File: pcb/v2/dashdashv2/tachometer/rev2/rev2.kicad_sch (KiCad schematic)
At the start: 182 parts, among them Q1 BSS138, Q2 BSS138, Q3 BSS138, Q4 BSS138, Q5 BSS138, Q6 BSS138, Q7 BSS138, U1 SK6812SIDE

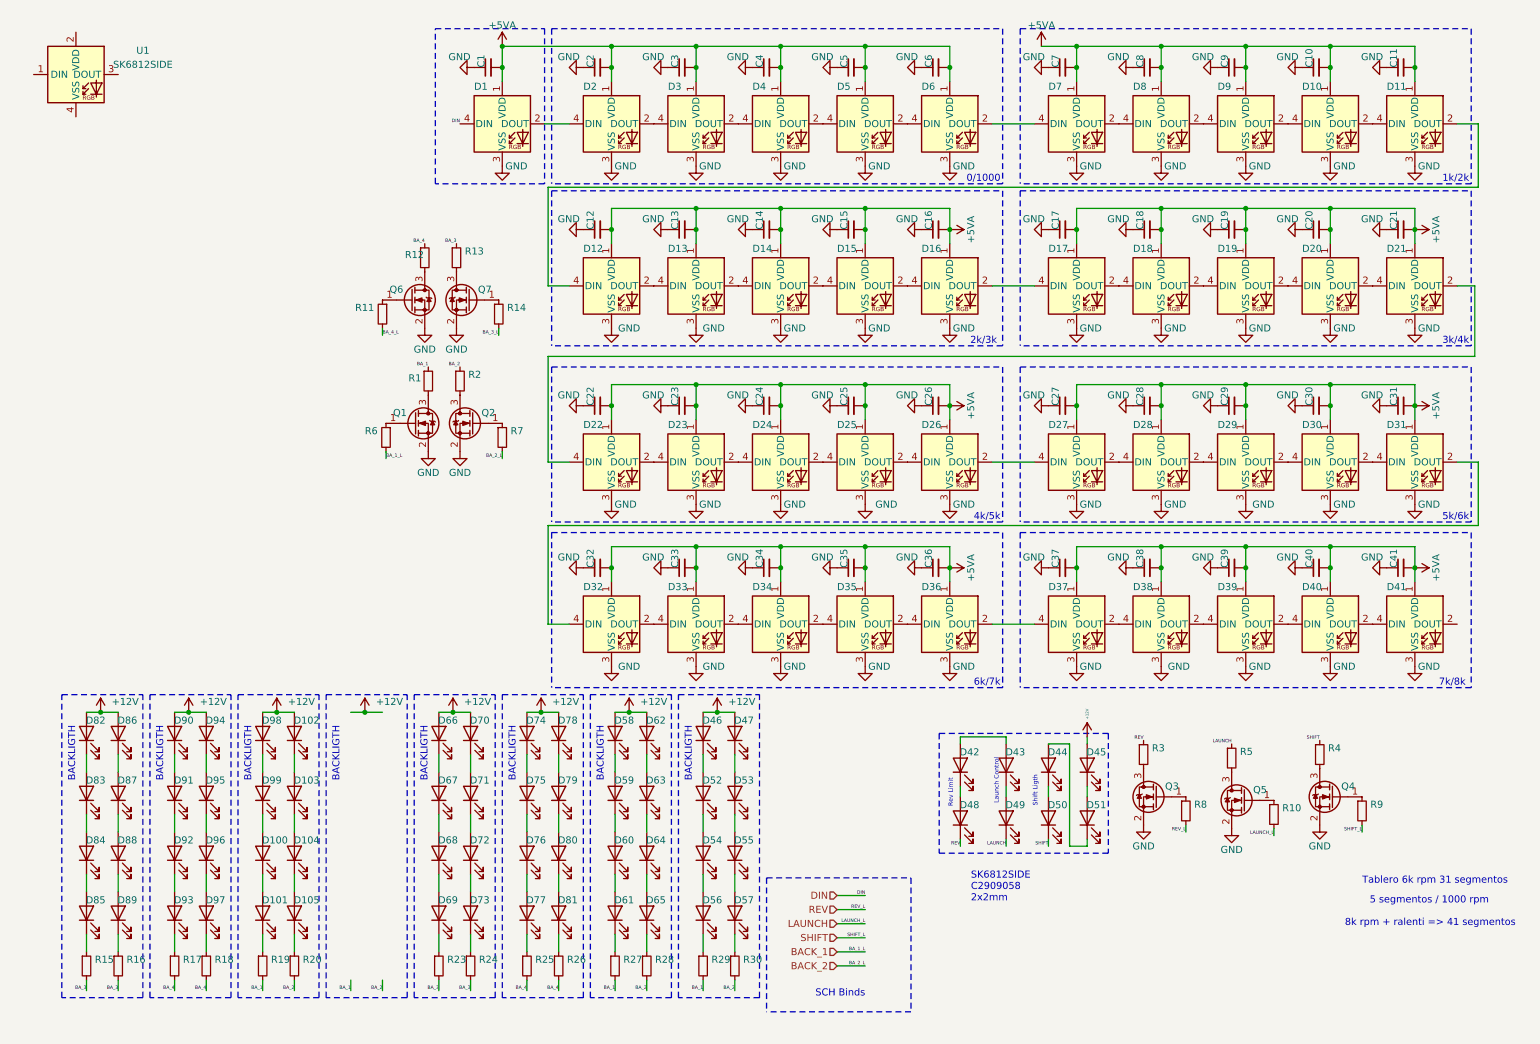
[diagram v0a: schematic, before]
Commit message: tach v2, routing & 3D
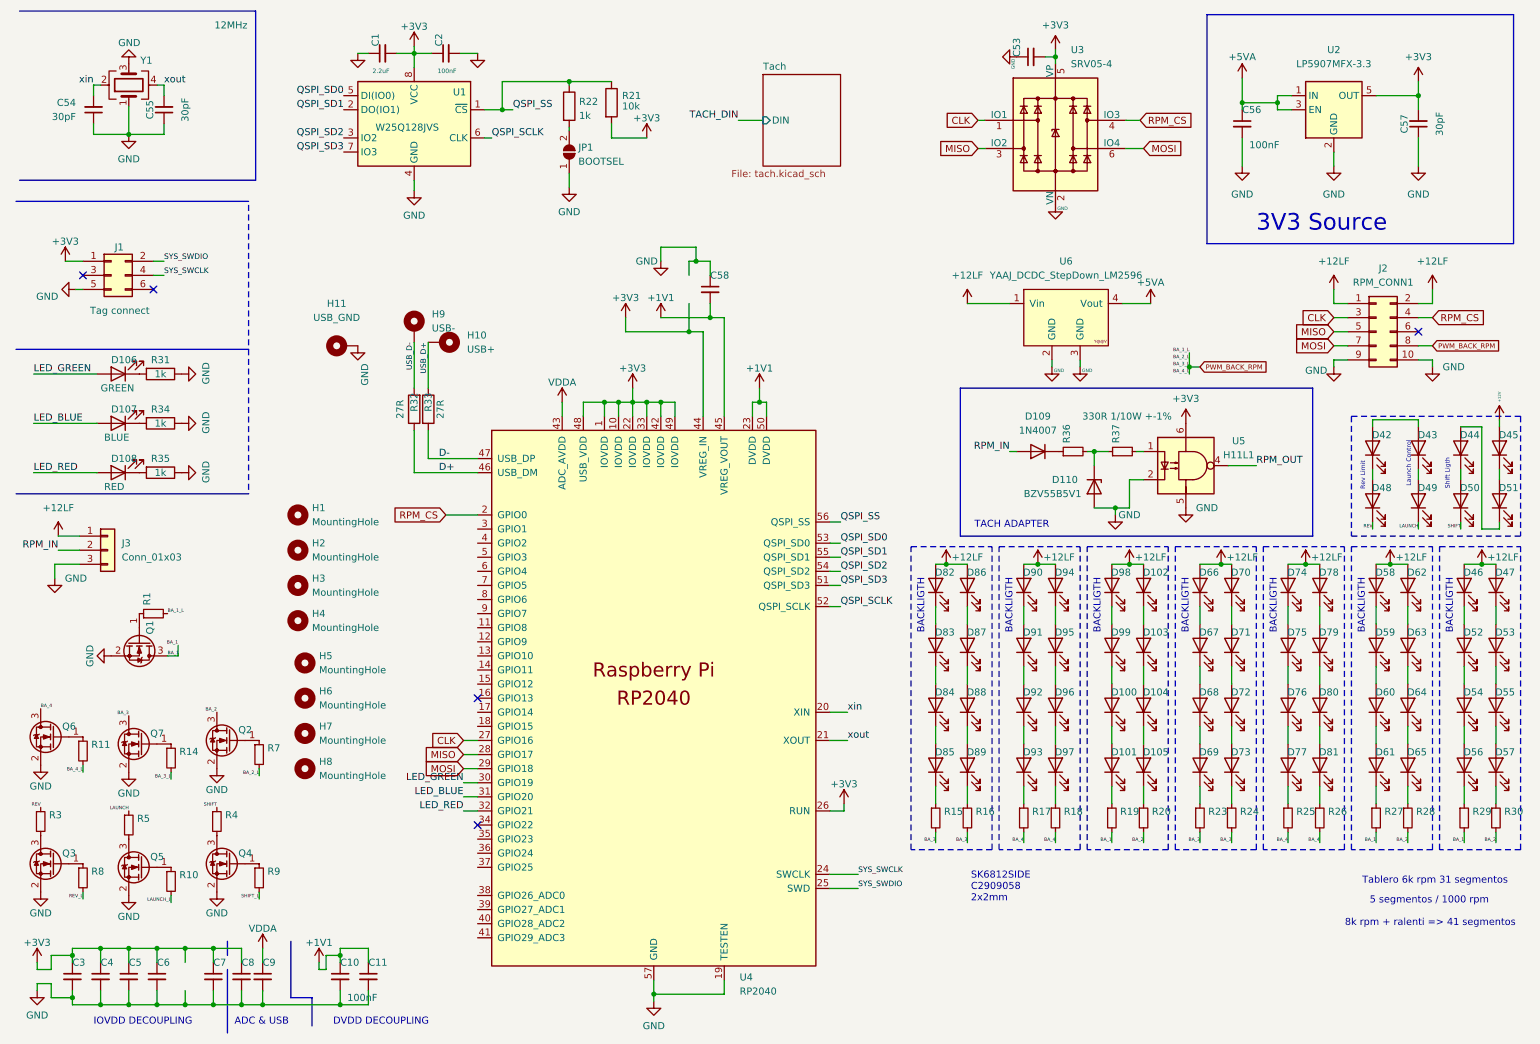
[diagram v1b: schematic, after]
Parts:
- removed C12, C13, C14, C15, C16, C17, C18, C19, C20, C21, C22, C23, C24, C25, C26, C27, C28, C29, C30, C31, C32, C33, C34, C35, C36, C37, C38, C39, C40, C41: 100nF, Capacitor_SMD:C_0805_2012Metric, symbol Device:C_Small
- removed D1, D10, D11, D12, D13, D14, D15, D16, D17, D18, D19, D2, D20, D21, D22, D23, D24, D25, D26, D27, D28, D29, D3, D30, D31, D32, D33, D34, D35, D36, D37, D38, D39, D4, D40, D41, D5, D6, D7, D8, D9: WS2812B, LED_SMD:LED_Cree-PLCC4_2x2mm_CW, symbol LED:WS2812B
- removed R12, R13, R2, R6: 1k 1/10W +-1%, Resistor_SMD:R_0603_1608Metric, symbol Device:R_Small
- removed U1: SK6812SIDE, symbol dashdashv2:SK6812SIDE
- added C53, C56: 100nF, Capacitor_SMD:C_0603_1608Metric, symbol Device:C_Small
- added C54, C55, C57: 30pF, Capacitor_SMD:C_0603_1608Metric, symbol Device:C_Small
- added C58: 2.2uF, Capacitor_SMD:C_0603_1608Metric, symbol Device:C_Small
- added D106: GREEN, LED_SMD:LED_0603_1608Metric, symbol Device:LED
- added D107: BLUE, LED_SMD:LED_0603_1608Metric, symbol Device:LED
- added D108: RED, LED_SMD:LED_0603_1608Metric, symbol Device:LED
- added D109: 1N4007, Diode_THT:D_DO-41_SOD81_P7.62mm_Horizontal, symbol Diode:1N4007
- added D110: BZV55B5V1, Diode_SMD:D_MiniMELF, symbol Diode:BZV55B5V1
- added H1, H2, H3, H4, H5, H6, H7, H8: MountingHole, MountingHole:MountingHole_2.2mm_M2_Pad, symbol Mechanical:MountingHole
- added H10: USB+, TestPoint:TestPoint_Pad_D1.5mm, symbol Mechanical:MountingHole_Pad
- added H11: USB_GND, TestPoint:TestPoint_Pad_D1.5mm, symbol Mechanical:MountingHole_Pad
- added H9: USB-, TestPoint:TestPoint_Pad_D1.5mm, symbol Mechanical:MountingHole_Pad
- added J1: Tag connect, Connector:Tag-Connect_TC2030-IDC-FP_2x03_P1.27mm_Vertical, symbol Connector_Generic:Conn_02x03_Odd_Even
- added J2: RPM_CONN1, Connector_PinHeader_1.27mm:PinHeader_2x05_P1.27mm_Vertical, symbol Connector_Generic:Conn_02x05_Odd_Even
- added J3: Conn_01x03, Connector_PinHeader_2.54mm:PinHeader_1x03_P2.54mm_Vertical, symbol Connector_Generic:Conn_01x03
- added JP1: BOOTSEL, Jumper:SolderJumper-2_P1.3mm_Open_TrianglePad1.0x1.5mm, symbol Jumper:SolderJumper_2_Open
- added R21: 10k, Resistor_SMD:R_0603_1608Metric, symbol Device:R
- added R22, R31, R34, R35: 1k, Resistor_SMD:R_0603_1608Metric, symbol Device:R
- added R32, R33: 27R, Resistor_SMD:R_0603_1608Metric, symbol Device:R
- added R36: 1k 1/10W +-1%, Resistor_SMD:R_0603_1608Metric, symbol Device:R_Small
- added R37: 330R 1/10W +-1%, Resistor_SMD:R_0603_1608Metric, symbol Device:R_Small
- added U1: W25Q128JVS, Package_SO:SOIC-8_5.23x5.23mm_P1.27mm, symbol Memory_Flash:W25Q128JVS
- added U2: LP5907MFX-3.3, Package_TO_SOT_SMD:SOT-23-5, symbol Regulator_Linear:LP5907MFX-3.3
- added U3: SRV05-4, Package_TO_SOT_SMD:SOT-23-6, symbol Power_Protection:SRV05-4
- added U4: RP2040, Package_DFN_QFN:QFN-56-1EP_7x7mm_P0.4mm_EP3.2x3.2mm, symbol rp2040:RP2040
- added U5: H11L1, Package_DIP:DIP-6_W7.62mm_Socket, symbol Isolator:H11L1
- added U6: YAAJ_DCDC_StepDown_LM2596, dashdash_lib:YAAJ_DCDC_StepDown_LM2596, symbol dashdashv2:YAAJ_DCDC_StepDown_LM2596
- added Y1: 12MHz, Crystal:Crystal_SMD_3225-4Pin_3.2x2.5mm, symbol Device:Crystal_GND24
- C1: value 100nF -> 2.2uF; footprint Capacitor_SMD:C_0805_2012Metric -> Capacitor_SMD:C_0603_1608Metric; LCSC C49678 -> (none)
- C10, C11, C2, C3, C4, C5, C6, C7, C8, C9: footprint Capacitor_SMD:C_0805_2012Metric -> Capacitor_SMD:C_0603_1608Metric; LCSC C49678 -> (none)
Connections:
- net BACK_2 is gone; now on net PWM_BACK_RPM: R7.2
- net BA_3_L is gone; now on net PWM_BACK_RPM: R14.2
- net BA_4_L is gone; now on net PWM_BACK_RPM: R11.2
- net +12V: no longer D102.2 (A), D46.2 (A), D47.2 (A), D58.2 (A), D62.2 (A), D66.2 (A), D70.2 (A), D74.2 (A), D78.2 (A), D82.2 (A), D86.2 (A), D90.2 (A), D94.2 (A), D98.2 (A)
- net +5VA: now also C56.1, U2.1 (IN), U2.3 (EN), U6.4 (Vout); no longer C1.2, C10.2, C11.2, C2.2, C3.2, C4.2, C5.2, C6.2, C7.2, C8.2, C9.2
- net BA_1: now also Q1.3 (D); no longer R1.1
- net BA_2: now also Q2.3 (D)
- net BA_3: now also Q7.3 (D)
- net BA_4: now also Q6.3 (D)
- net GND: now also C10.2, C11.2, C2.2, C3.2, C4.2, C5.2, C6.2, C7.2, C8.2, C9.2, C53.1, C54.1, C55.1, C56.2, C57.1, C58.1, D110.2 (A), H11.1, J1.5 (Pin_5), J2.10 (Pin_10), J2.9 (Pin_9), J3.3 (Pin_3), JP1.1 (A), R31.1, R34.1, R35.1, U1.4 (GND), U2.2 (GND), U3.2 (VN), U4.19 (TESTEN), U4.57 (GND), U5.2, U5.5, U6.2 (GND), U6.3 (GND), Y1.1, Y1.3; no longer C10.1, C11.1, C2.1, C3.1, C4.1, C5.1, C6.1, C7.1, C8.1, C9.1
- net LAUNCH: no longer R10.2
- net REV: no longer R8.2
- net SHIFT: no longer R9.2
- net at Q1.1 (G): now also R1.1
- net PWM_BACK_RPM: now reaches R1.2
- net PWM_BACK_RPM: now also J2.8 (Pin_8); no longer Q1.3 (D)
- new net: JP1.2 (B), R22.2
- new net: D109.1 (K), R36.1
- new net: D108.1 (K), R35.2
- new net: D110.1 (K), R36.2, R37.1
- new net: R37.2, U5.1
- new net: D107.1 (K), R34.2
- new net: D106.1 (K), R31.2
- new net +12LF: D102.2 (A), D46.2 (A), D47.2 (A), D58.2 (A), D62.2 (A), D66.2 (A), D70.2 (A), D74.2 (A), D78.2 (A), D82.2 (A), D86.2 (A), D90.2 (A), D94.2 (A), D98.2 (A), J2.1 (Pin_1), J2.2 (Pin_2), J3.1 (Pin_1), U6.1 (Vin)
- new net +1V1: C10.1, C11.1, C58.2, U4.23 (DVDD), U4.45 (VREG_VOUT), U4.50 (DVDD)
- new net +3V3: C1.2, C2.1, C3.1, C4.1, C5.1, C53.2, C57.2, C6.1, C7.1, C8.1, J1.1 (Pin_1), R21.2, U1.8 (VCC), U2.5 (OUT), U3.5 (VP), U4.1 (IOVDD), U4.10 (IOVDD), U4.22 (IOVDD), U4.26 (RUN), U4.33 (IOVDD), U4.42 (IOVDD), U4.44 (VREG_IN), U4.48 (USB_VDD), U4.49 (IOVDD), U5.6
- new net CLK: J2.3 (Pin_3), U3.1 (IO1), U4.27 (GPIO16)
- new net D+: R32.1, U4.46 (USB_DM)
- new net D-: R33.2, U4.47 (USB_DP)
- new net LAUNCH_L: R10.2
- new net LED_BLUE: D107.2 (A), U4.31 (GPIO20)
- new net LED_GREEN: D106.2 (A), U4.30 (GPIO19)
- new net LED_RED: D108.2 (A), U4.32 (GPIO21)
- new net MISO: J2.5 (Pin_5), U3.3 (IO2), U4.28 (GPIO17)
- new net MOSI: J2.7 (Pin_7), U3.6 (IO4), U4.29 (GPIO18)
- new net QSPI_SCLK: U1.6 (CLK), U4.52 (QSPI_SCLK)
- new net QSPI_SD0: U1.5 (DI(IO0)), U4.53 (QSPI_SD0)
- new net QSPI_SD1: U1.2 (DO(IO1)), U4.55 (QSPI_SD1)
- new net QSPI_SD2: U1.3 (IO2), U4.54 (QSPI_SD2)
- new net QSPI_SD3: U1.7 (IO3), U4.51 (QSPI_SD3)
- new net QSPI_SS: R21.1, R22.1, U1.1 (~{CS}), U4.56 (QSPI_SS)
- new net REV_L: R8.2
- new net RPM_CS: J2.4 (Pin_4), U3.4 (IO3), U4.2 (GPIO0)
- new net RPM_IN: D109.2 (A), J3.2 (Pin_2)
- new net RPM_OUT: U5.4
- new net SHIFT_L: R9.2
- new net SYS_SWCLK: J1.4 (Pin_4), U4.24 (SWCLK)
- new net SYS_SWDIO: J1.2 (Pin_2), U4.25 (SWD)
- new net USB_D+: H10.1, R33.1
- new net USB_D-: H9.1, R32.2
- new net VDDA: C9.1, U4.43 (ADC_AVDD)
- new net xin: C54.2, U4.20 (XIN), Y1.2
- new net xout: C55.2, U4.21 (XOUT), Y1.4
- no-connect marks 0 -> 5
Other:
- added sheet Tach (tach.kicad_sch)
- note added: "3V3 Source"
- note added: "ADC & USB"
- note added: "DVDD DECOUPLING"
- note added: "IOVDD DECOUPLING"
- note added: "TACH ADAPTER"
- note removed: "0/1000"
- note removed: "1k/2k"
- note removed: "2k/3k"
- note removed: "3k/4k"
- note removed: "4k/5k"
- note removed: "5k/6k"
- note removed: "6k/7k"
- note removed: "7k/8k"
- note removed: "SCH Binds"
- moved on the sheet: D100, D101, D102, D103, D104, D105, D42, D43, D44, D45, D46, D47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
